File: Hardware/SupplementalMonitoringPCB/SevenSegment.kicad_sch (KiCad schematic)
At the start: 41 parts, among them U1 SN74HC595N, U2 SN74HC595N, U3 SN74HC595N, U4 SN74HC595N

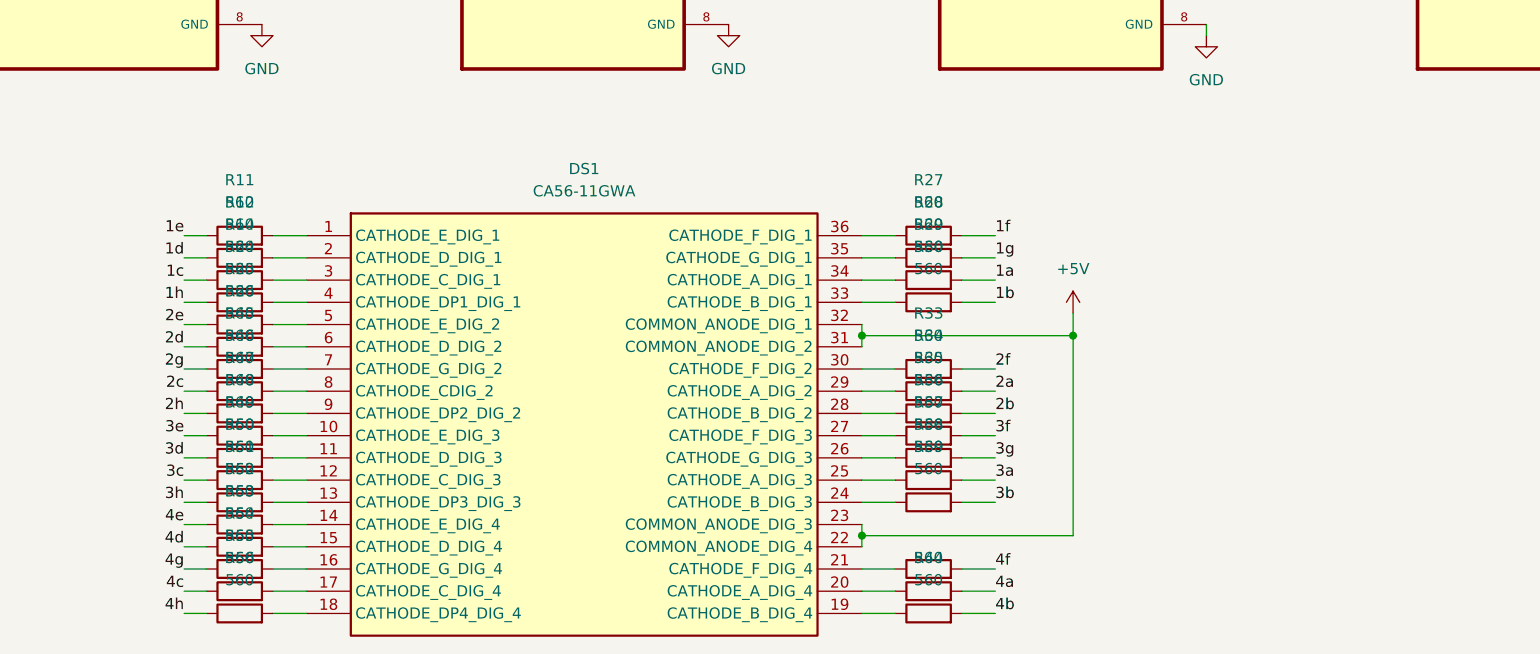
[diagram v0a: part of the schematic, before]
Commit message: labels
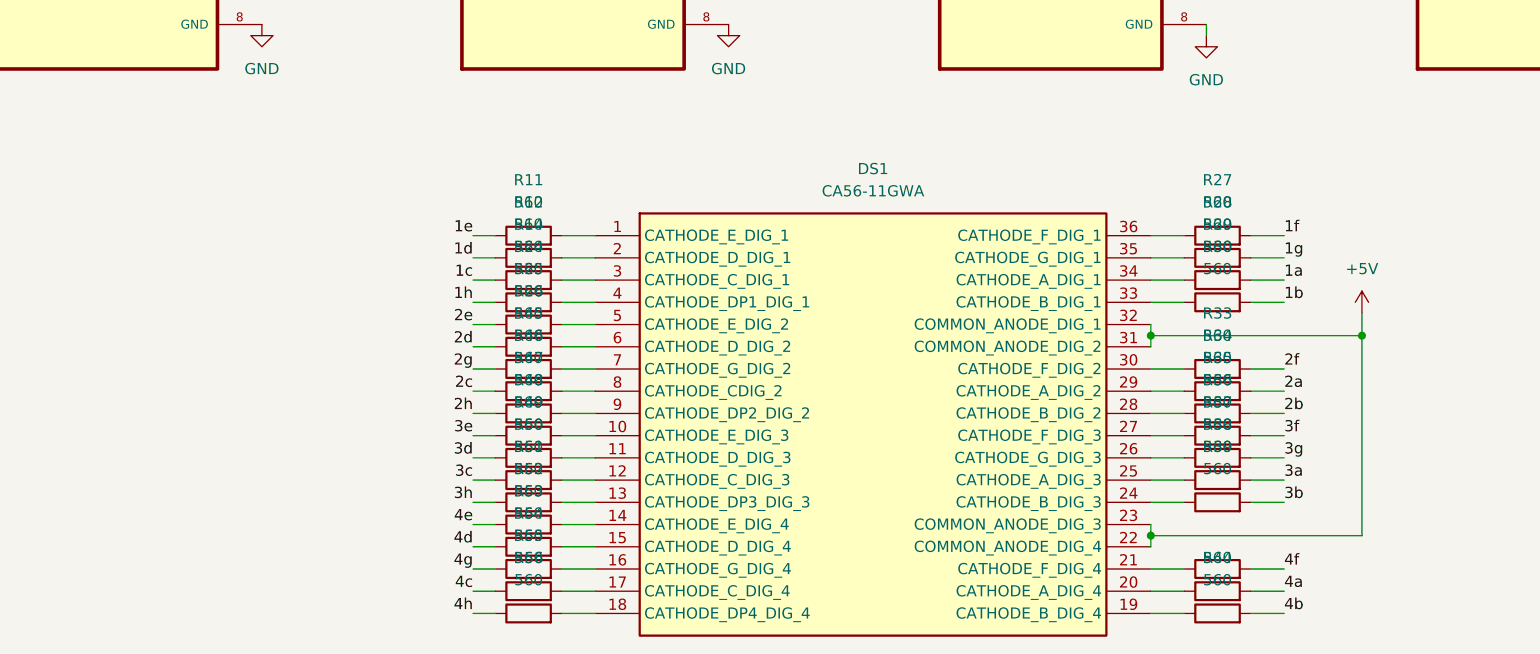
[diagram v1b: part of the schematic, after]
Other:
- moved on the sheet: DS1, R11, R12, R14, R24, R25, R26, R27, R28, R29, R30, R33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
